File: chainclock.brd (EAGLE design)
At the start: 60 x 40 mm, 16 parts

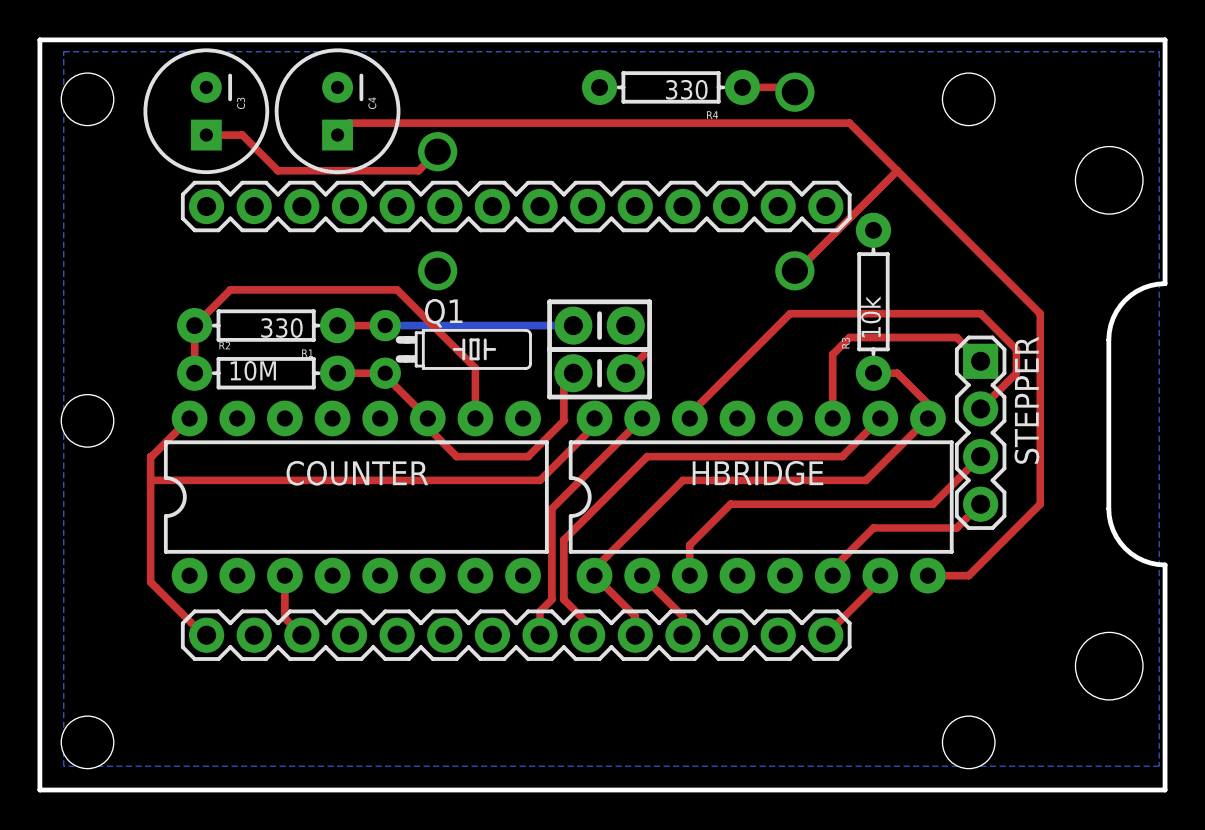
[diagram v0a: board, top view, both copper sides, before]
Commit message: Move some stuff around
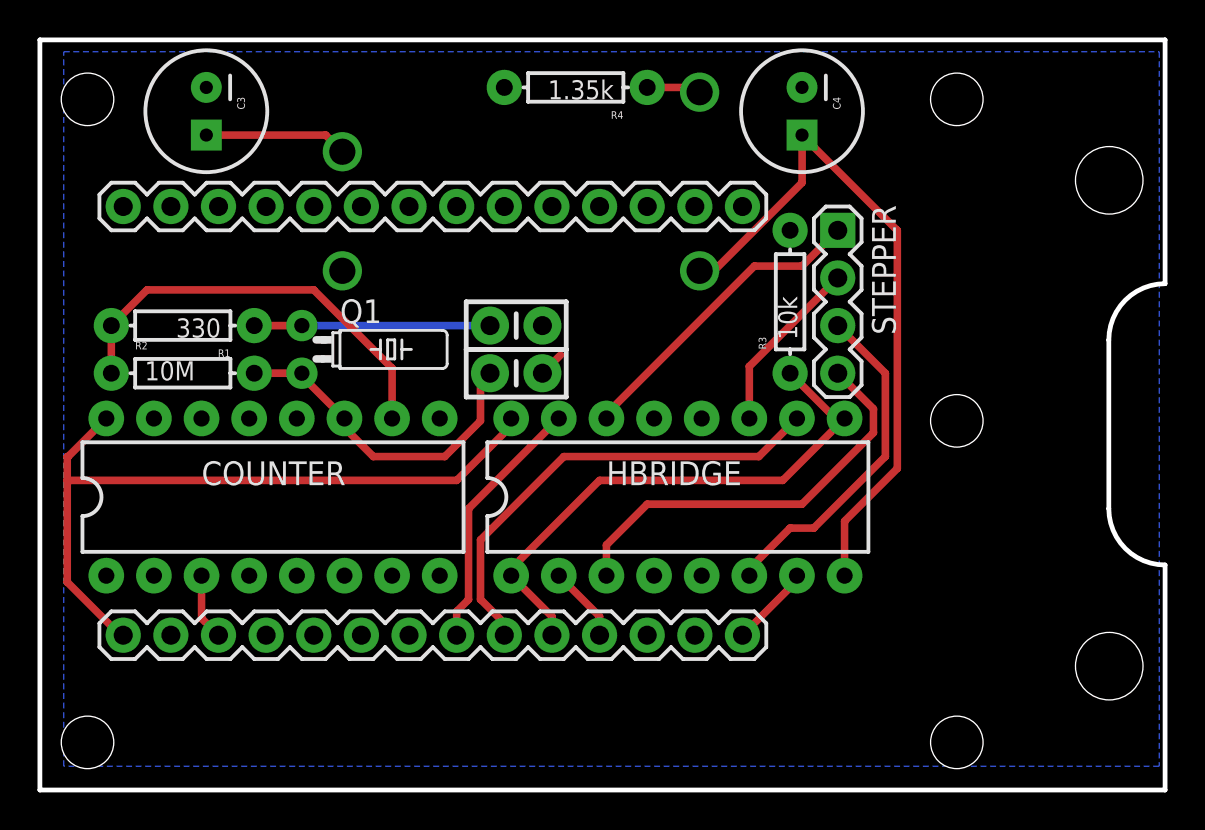
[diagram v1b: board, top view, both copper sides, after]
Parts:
- removed FRAME1: FRAME-LETTER, SparkFun-Aesthetics:CREATIVE_COMMONS
- R4: value 330 -> 1.35k
- moved C4 24.8 mm to (40.6, 36.2)
- moved STEPPER 10.3 mm to (42.5, 29.8)
- moved R4 5.08 mm to (28.6, 37.5)
- moved U$1 5.08 mm to (14.6, 38.7)
- moved ARDUNOFIO 4.45 mm to (38.7, 6.99)
- moved C1 4.45 mm to (25.4, 22.2)
- moved C2 4.45 mm to (25.4, 24.8)
- moved COUNTER 4.45 mm to (12.4, 15.6)
- moved HBRIDGE 4.45 mm to (34.0, 15.6)
- moved R3 4.45 mm to (40.0, 26.0)
- moved R1 4.44 mm to (7.62, 24.8)
- moved R2 4.44 mm to (7.62, 22.2)
- moved Q1 4.44 mm to (14.0, 23.5)
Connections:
- net 1Y: now also STEPPER.4; no longer STEPPER.3
- net 2Y: now also STEPPER.3; no longer STEPPER.4
- net 3Y: now also STEPPER.2; no longer STEPPER.1
- net 4Y: now also STEPPER.1; no longer STEPPER.2
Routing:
- net VDD12: track 67.3 -> 36.7 mm
- net 2Y: track 9.68 -> 18.1 mm
- net 4Y: track 24.6 -> 16.6 mm
- net VIN: track 13.5 -> 7.62 mm
- net 1Y: track 19.1 -> 22.3 mm
- net 3Y: track 12.2 -> 9.45 mm
- net EN: track 30.1 -> 29.6 mm
